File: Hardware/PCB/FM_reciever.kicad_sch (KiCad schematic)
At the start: 15 parts, among them U1 ${SIM.PARAMS}, U2 ${SIM.PARAMS}

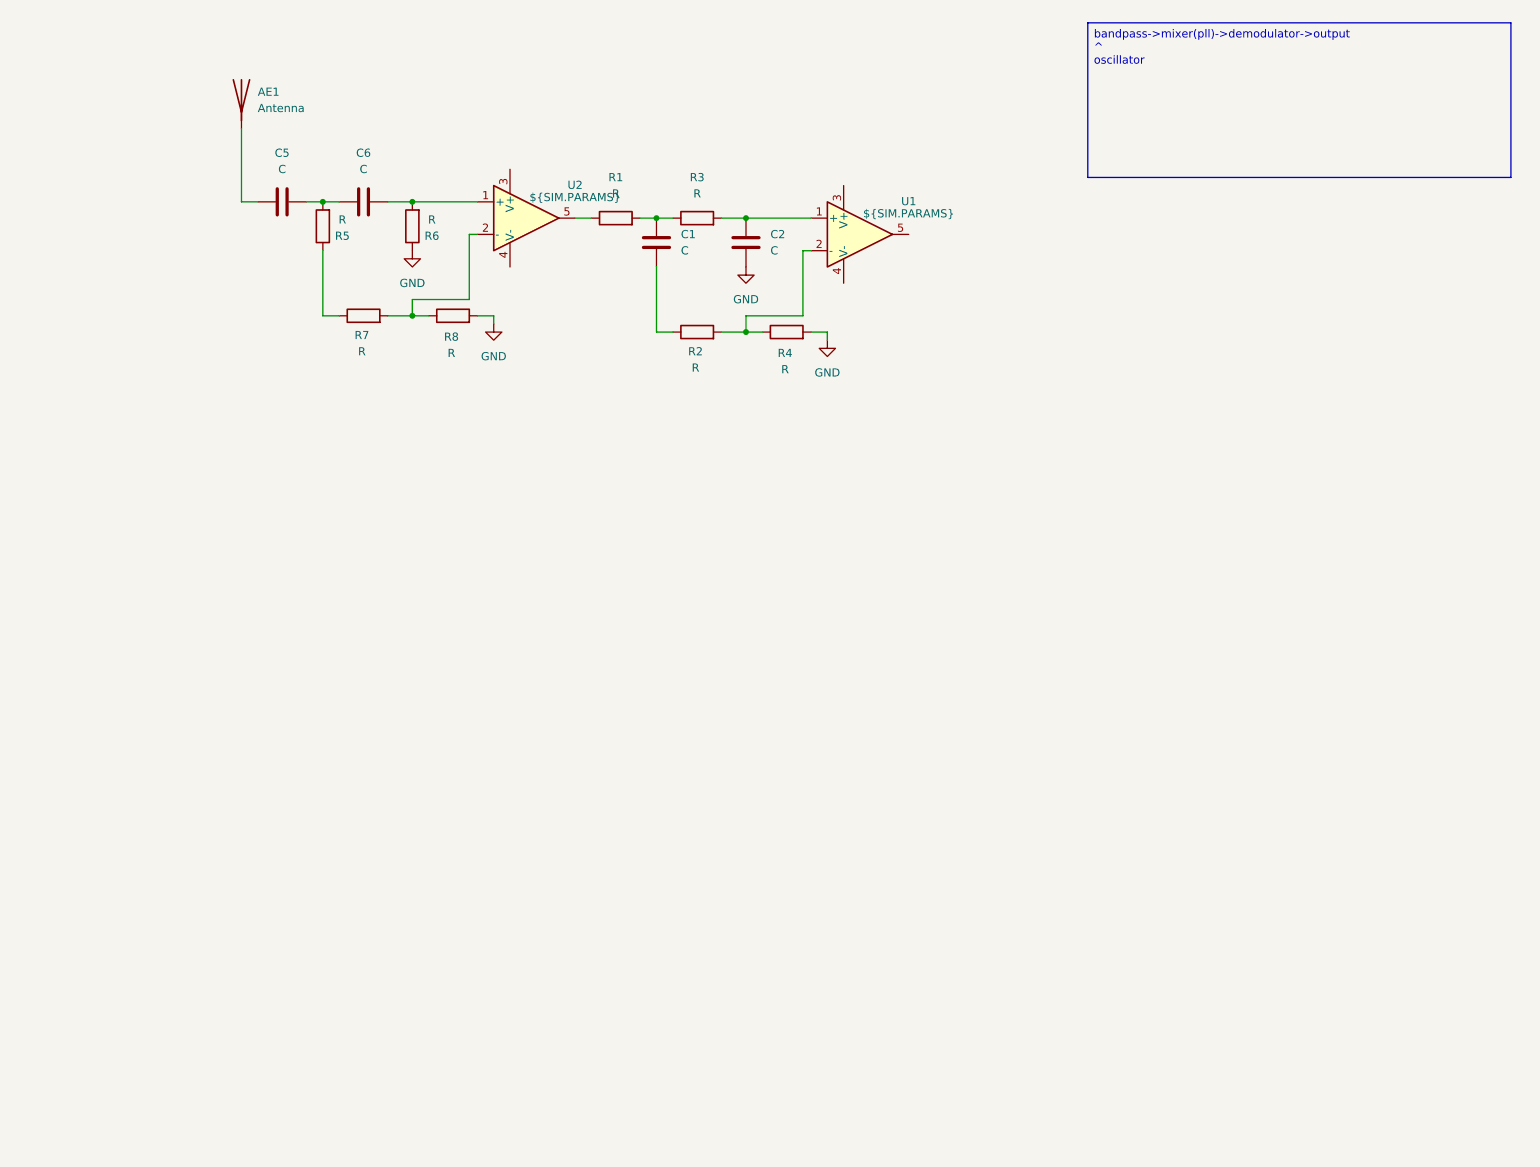
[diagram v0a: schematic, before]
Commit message: mixer and bandpass worked out
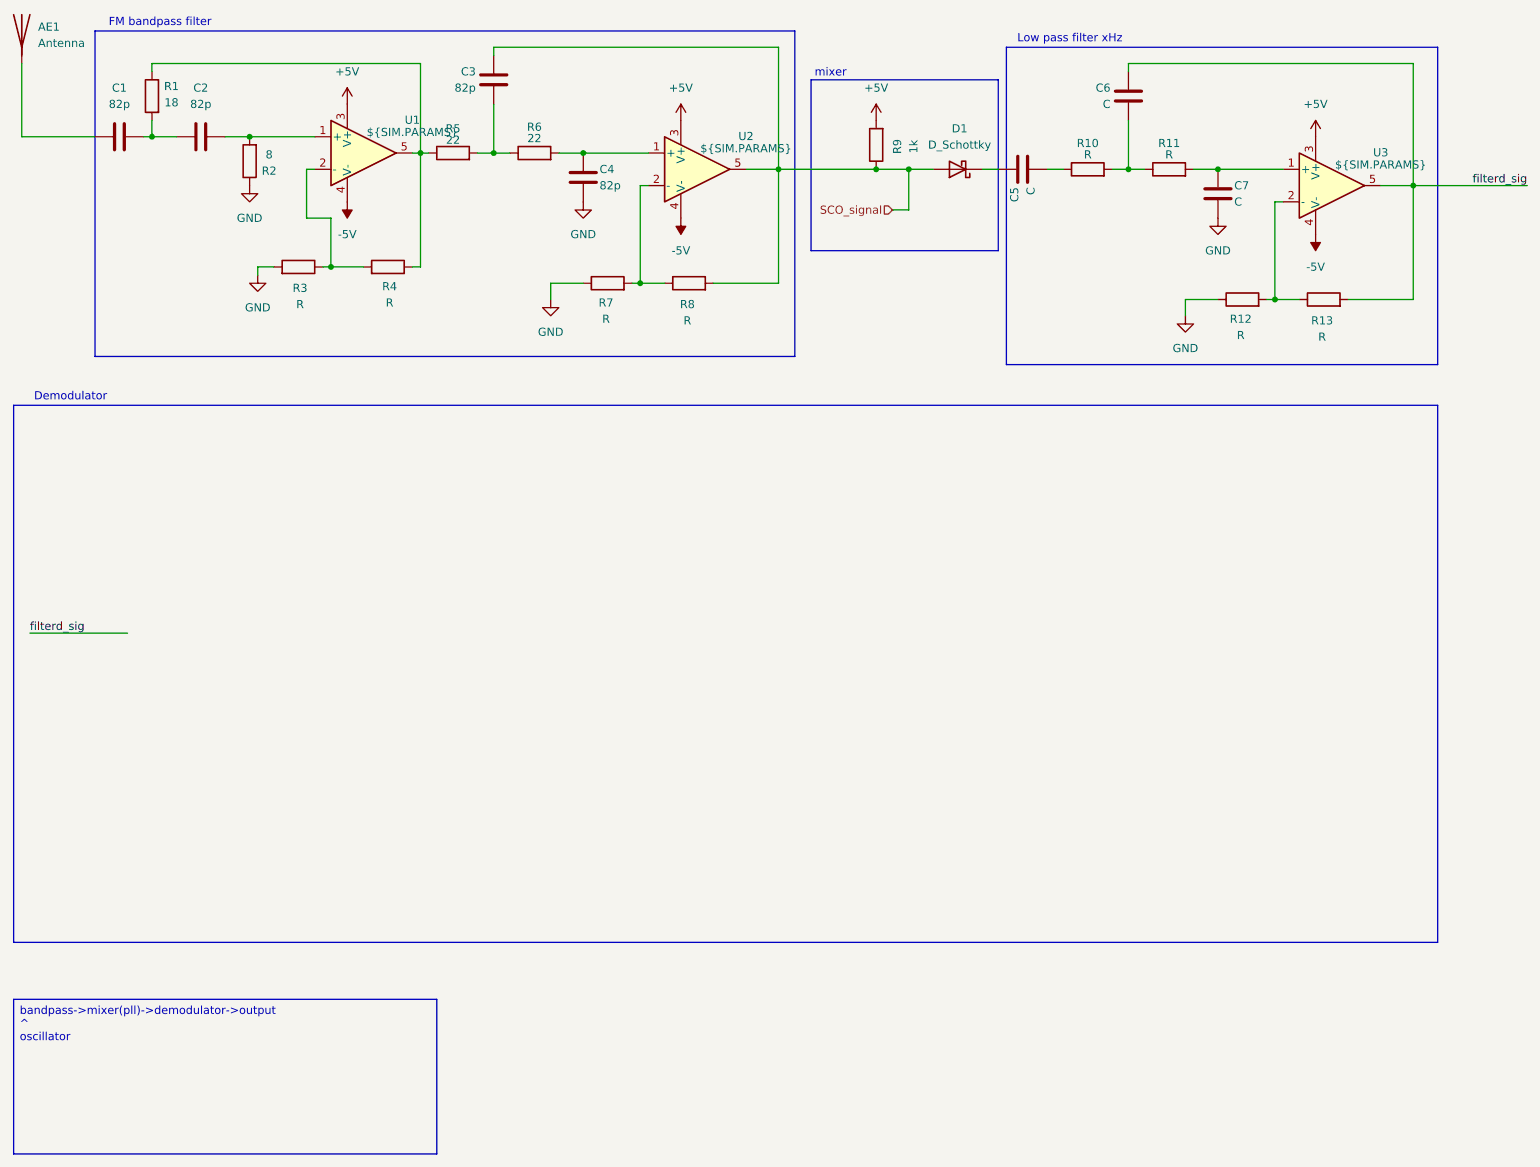
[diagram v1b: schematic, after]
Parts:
- added C5, C6, C7: C, symbol Device:C
- added D1: D_Schottky, symbol Device:D_Schottky
- added R10, R11, R12, R13: R, symbol Device:R
- added R9: 1k, symbol Device:R
- added U3: ${SIM.PARAMS}, symbol Simulation_SPICE:OPAMP
- C1: renamed from C5; value C -> 82p
- C2: renamed from C6; value C -> 82p
- C3: renamed from C1; value C -> 82p
- C4: renamed from C2; value C -> 82p
- R1: renamed from R5; value R -> 18
- R2: renamed from R6; value R -> 8
- R5: renamed from R1; value R -> 22
- R6: renamed from R3; value R -> 22
- renumbered R8 to R3, R7 to R4, R2 to R7, R4 to R8, U2 to U1, U1 to U2
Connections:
- net GND: now also R7.1, C7.2, R12.1; no longer R8.2
- net +5V: now reaches U1.3 (V+)
- net +5V: now also U2.3 (V+), R9.2, U3.3 (V+)
- net -5V: now reaches U1.4 (V-)
- net -5V: now also U2.4 (V-), U3.4 (V-)
- net at R5.1, U1.5: now also R1.1, R4.1
- net SCO_signal: now reaches C3.2
- net SCO_signal: now also R8.2, U2.5, D1.2 (A), R9.1; no longer R7.1
- new net: C5.2, D1.1 (K)
- new net: R12.2, R13.1, U3.2 (-)
- new net: C7.1, R11.2, U3.1 (+)
- new net: C6.1, R10.2, R11.1
- new net: C5.1, R10.1
- new net filterd_sig: C6.2, R13.2, U3.5
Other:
- note added: "Demodulator"
- note added: "FM bandpass filter"
- note added: "Low pass filter xHz"
- note added: "mixer"
- moved on the sheet: AE1, C1, C2, C3, C4, R1, R2, R3, R4, R5, R6, R7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
